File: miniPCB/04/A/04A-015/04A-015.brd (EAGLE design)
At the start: 28 parts

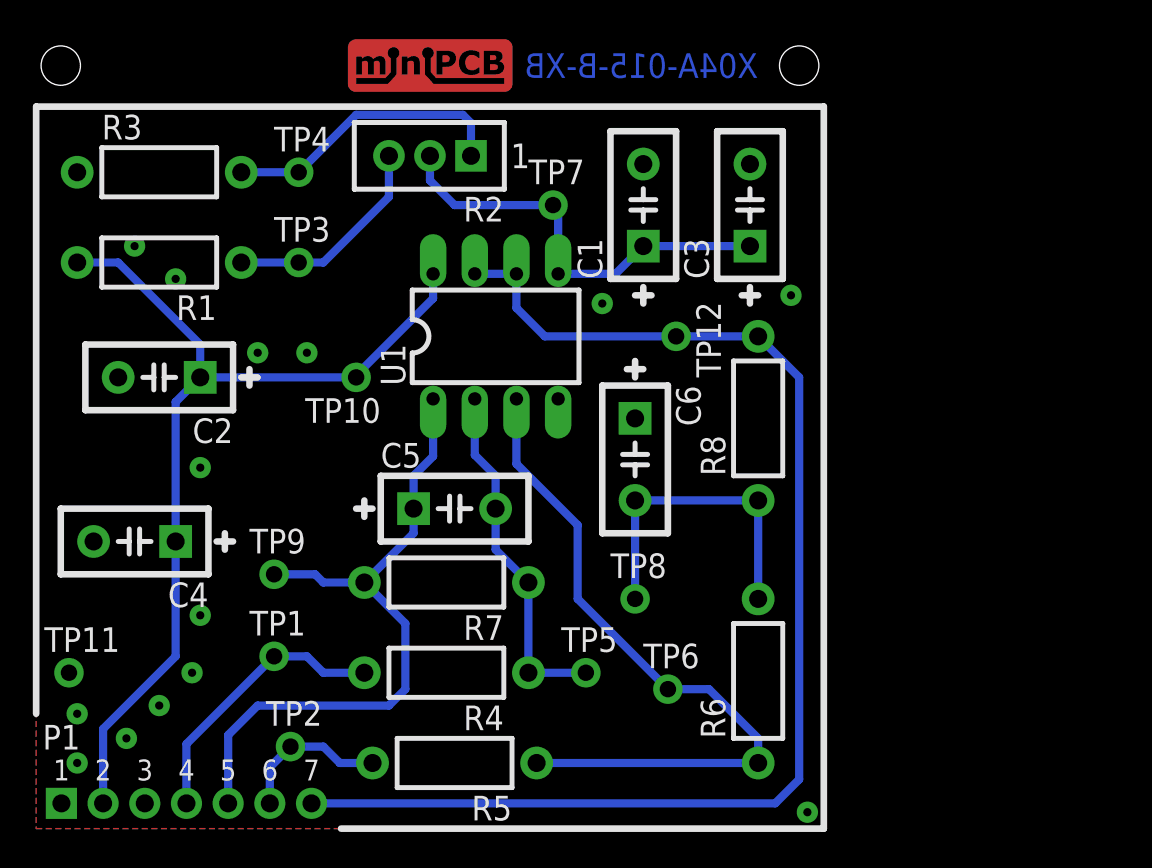
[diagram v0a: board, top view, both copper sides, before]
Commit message: NM.07SEP2023
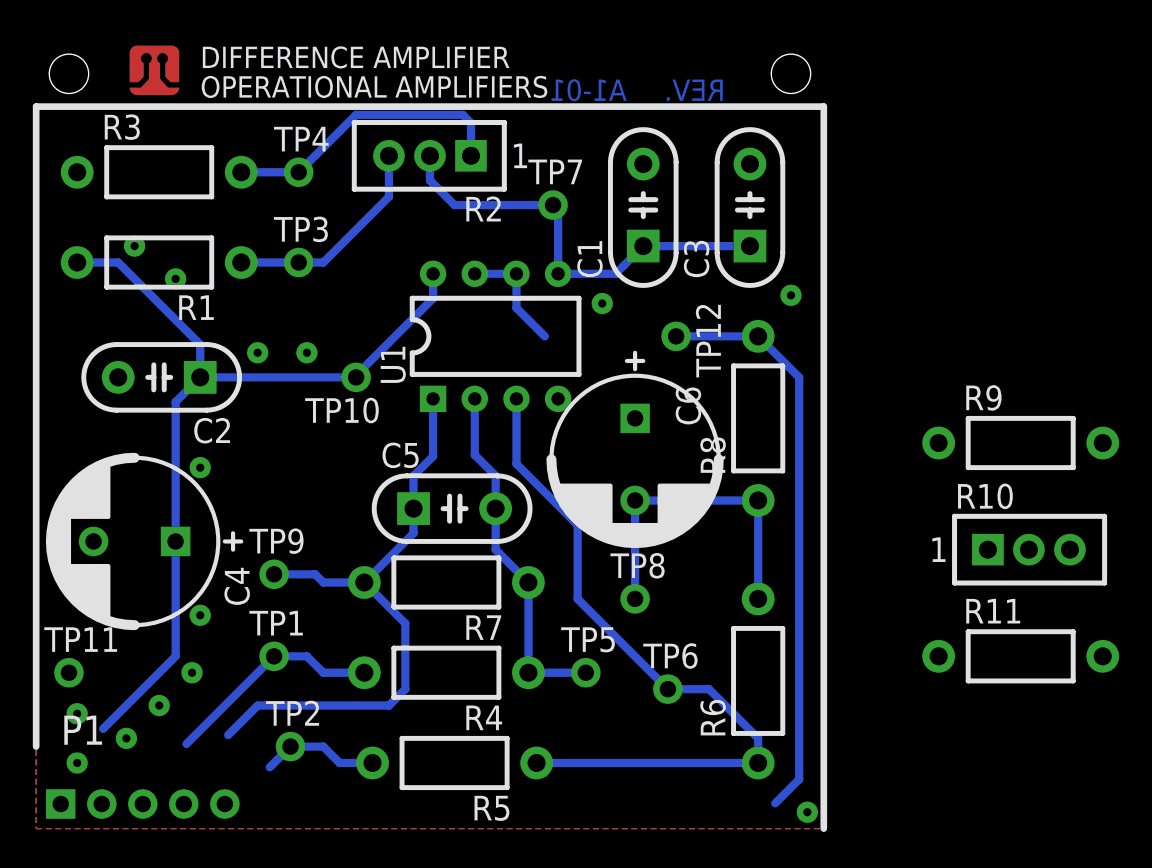
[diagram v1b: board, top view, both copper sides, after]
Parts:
- removed P1-: (no value), minipcb:MINIPCB_7P_50X50
- added P1: (no value), minipcb:PINS_1X5
- added R10: (no value), minipcb:TRIM_0100
- added R11, R9: (no value), minipcb:0207/10
- added U$1: MINIPCB_50X50, minipcb:MINIPCB_0P_50X50MM
- C4, C6: device minipcb:C050-024X044 -> minipcb:C5MM
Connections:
- new net N$5: R8.2, TP12.1
- new net N$6: R10.2, R11.2
- net GND: now also C4.-, C6.+, P1.1; no longer C4.2, C6.1, P1-.1
- net IN: now also P1.4; no longer P1-.4
- net N$2: now also R9.1, U1.6, U1.7; no longer C6.2, R6.2, R8.1, TP8.1
- net N$4: no longer P1-.6
- net NC: now also P1.3; no longer P1-.3
- net OUT: now also P1.5, R10.1; no longer P1-.5
- net V+: now also C4.+, P1.2; no longer C4.1, P1-.2
- net VFB: now also R11.1
- net VREF: now also C6.-, R6.2, R8.1, R9.2, TP8.1; no longer P1-.7, R8.2, TP12.1, U1.6, U1.7
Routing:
- net VREF: track 78.4 -> 19.5 mm
- net N$5: track 0.00 -> 35.1 mm
- net N$2: track 19.5 -> 7.07 mm
- net V+: track 57.7 -> 53.2 mm
- net OUT: track 42.3 -> 38.1 mm
- net IN: track 17.1 -> 13.5 mm
- net N$4: track 9.40 -> 7.20 mm

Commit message: NM.15SEP2023
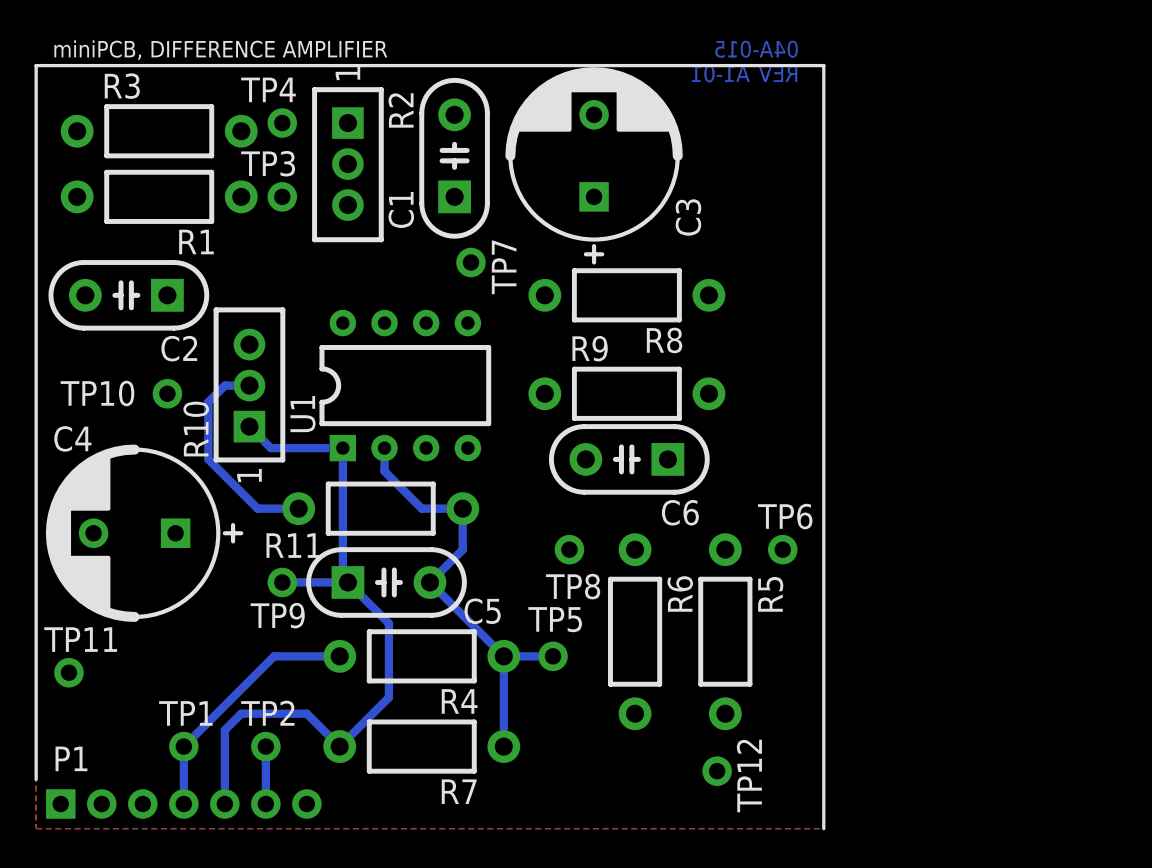
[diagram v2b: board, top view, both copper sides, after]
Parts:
- removed P1: (no value), minipcb:PINS_1X5
- added P2: (no value), minipcb:PINS_1X7
- C3: device minipcb:C050-024X044 -> minipcb:C5MM
- C6: device minipcb:C5MM -> minipcb:C050-024X044
- U$1: value MINIPCB_50X50 -> CLASSIC-50; device minipcb:MINIPCB_0P_50X50MM -> miniPCB_BOARDS:PCB50
- moved R10 45.6 mm to (14.0, 25.5), turned to 90 degrees
- moved R11 40.0 mm to (22.0, 20.5), turned to 180 degrees
- moved TP12 26.6 mm to (42.5, 4.50)
- moved R9 24.2 mm to (37.0, 27.5)
- moved R5 18.3 mm to (43.0, 13.0), turned to 270 degrees
- moved C1 11.9 mm to (26.5, 42.0)
- moved TP10 11.5 mm to (9.00, 27.5), turned to 270 degrees
- moved TP6 11.0 mm to (46.5, 18.0)
- moved R8 11.0 mm to (37.0, 33.5), turned to 180 degrees
- moved R7 10.1 mm to (24.5, 6.00)
- moved C3 9.96 mm to (35.0, 42.0)
- moved R6 8.08 mm to (37.5, 13.0), turned to 270 degrees
- moved TP1 7.78 mm to (10.0, 6.00)
- moved R2 7.76 mm to (20.0, 44.0), turned to 270 degrees
- moved U1 6.26 mm to (23.5, 28.0)
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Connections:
- net N$2 renamed VFBREF
- net N$3 renamed VPOS
- removed net IN: P1.4, R4.2, TP1.1
- removed net N$1: C1.1, C3.1, R2.2, TP7.1, U1.5
- removed net N$4: R5.2, TP2.1
- removed net N$5: R8.2, TP12.1
- new net IN+: P2.4, R4.2, TP1.1
- new net IN-: P2.6, R5.2, TP2.1
- new net OUTREF: P2.7, R8.2, TP12.1
- new net REF: C1.1, C3.+, R2.2, TP7.1, U1.5
- net GND: now also C3.-, C6.1, P2.1; no longer C3.2, C6.+, P1.1
- net NC: now also P2.3; no longer P1.3
- net OUT: now also P2.5; no longer P1.5
- net V+: now also P2.2; no longer P1.2
- net VREF: now also C6.2; no longer C6.-
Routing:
- net V+: track 53.2 -> 0.00 mm
- net VPOS: track 43.3 -> 0.00 mm
- net N$5: track 35.1 -> 0.00 mm
- net N$1: track 26.3 -> 0.00 mm
- net VREF: track 19.5 -> 0.00 mm
- net P1.1: track 17.7 -> 0.00 mm
- net IN+: track 0.00 -> 15.3 mm
- net IN: track 13.5 -> 0.00 mm
- net N$6: track 0.00 -> 13.2 mm
- net P1.3: track 13.2 -> 0.00 mm
- net N$4: track 7.20 -> 0.00 mm
- net VFBREF: track 7.07 -> 0.00 mm
- net VFB: track 21.5 -> 27.5 mm
- net OUT: track 38.1 -> 43.6 mm
- net IN-: track 0.00 -> 3.50 mm
